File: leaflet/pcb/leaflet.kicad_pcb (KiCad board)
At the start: 2 copper layers, 99.1 x 48.3 mm, 34 parts, among them J1 Conn_01x02, J2 Conn_01x02, J3 USB_B_Micro, J4 Conn_01x14_Male, J5 Conn_01x14_Male, Q1 NTZD3155C, Q2 NTZD3155C, U1 MCP16252-I_CH, U2 MCP1711, U3 EFM32HG322F64G-B-QFP48, U4 IP4220CZ6, U5 NRF24L01_Breakout

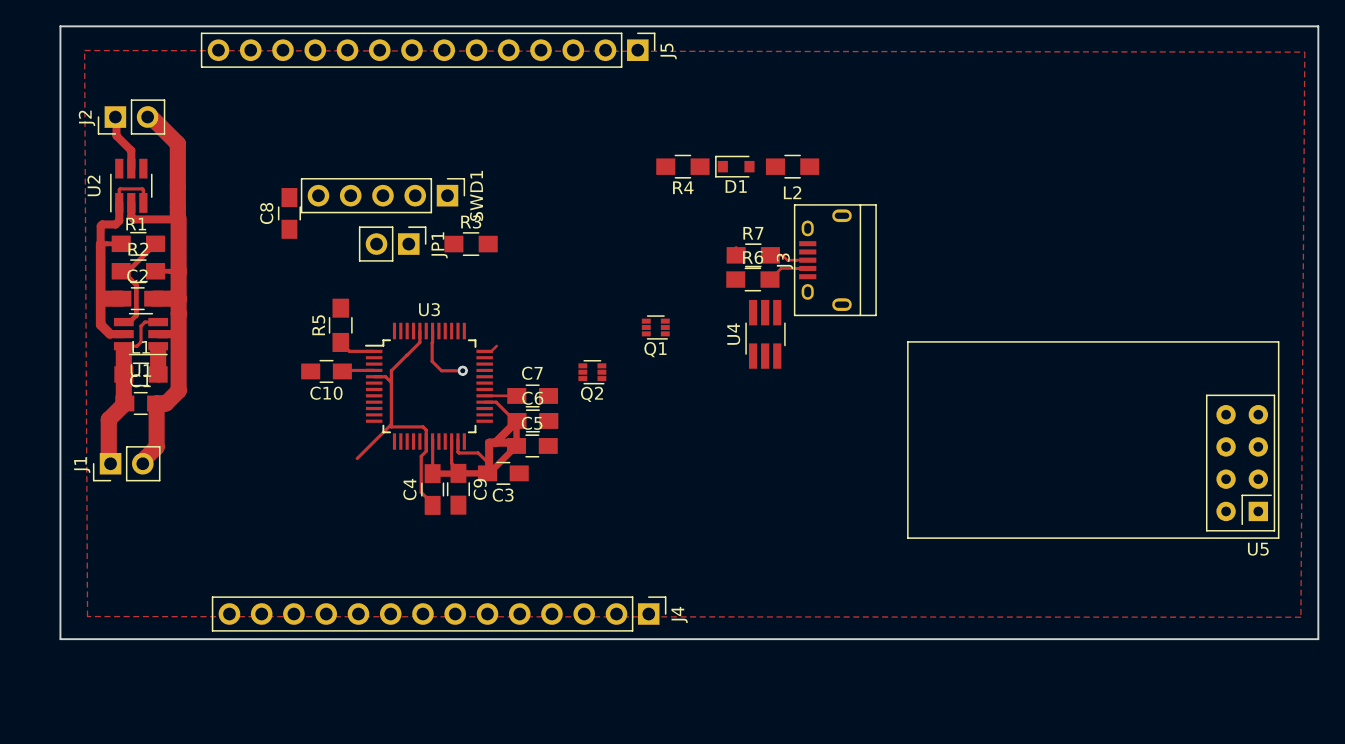
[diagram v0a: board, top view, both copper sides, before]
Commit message: stuff
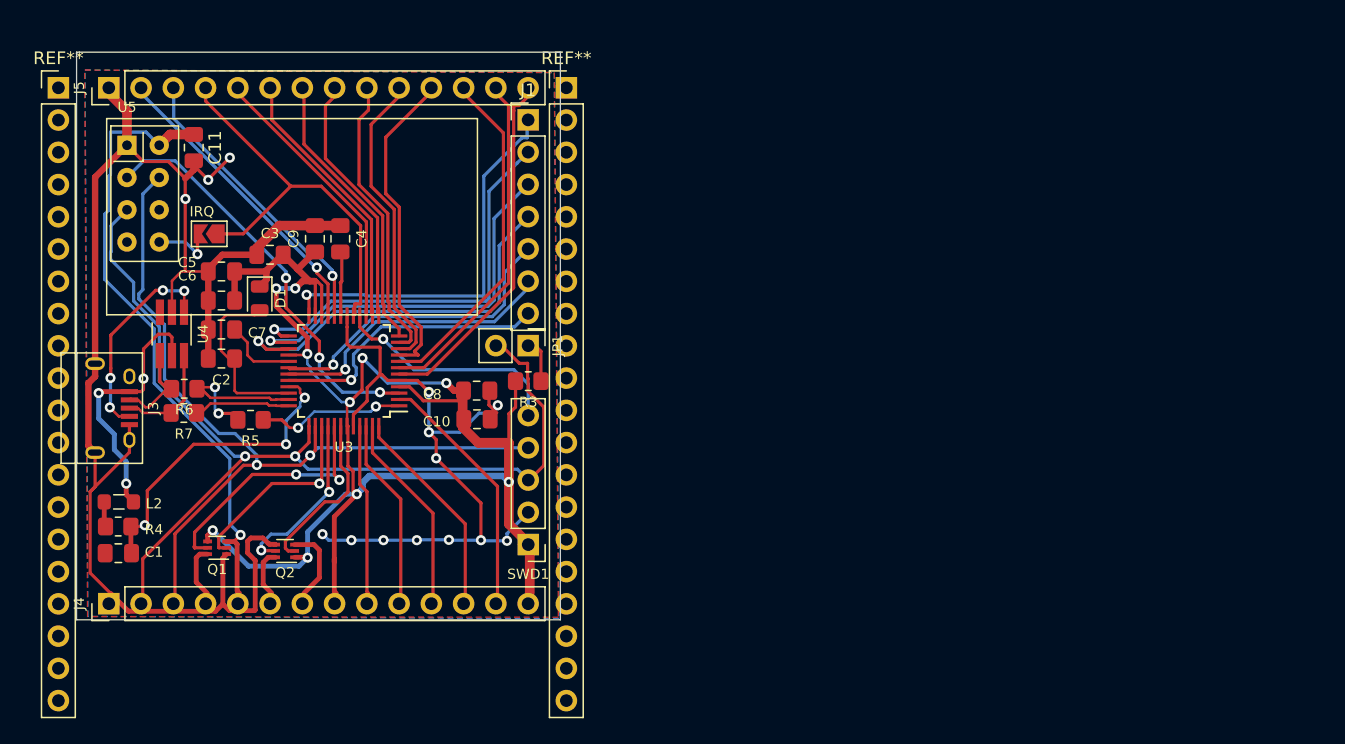
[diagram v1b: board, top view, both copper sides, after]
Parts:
- removed J2: Conn_01x02, Pin_Headers:Pin_Header_Straight_1x02_Pitch2.54mm
- removed L1: 4.7u, Inductors_SMD:L_0805_HandSoldering
- removed R1: 1.8M, Resistors_SMD:R_0805_HandSoldering
- removed R2: 1M, Resistors_SMD:R_0805_HandSoldering
- removed U1: MCP16252-I_CH, TO_SOT_Packages_SMD:SOT-23-6_Handsoldering
- removed U2: MCP1711, TO_SOT_Packages_SMD:SOT-23-6_Handsoldering
- added C11: 100n, Capacitor_SMD:C_0805_2012Metric_Pad1.18x1.45mm_HandSolder, F.Cu at (20.7, 19.7)
- added IRQ: Jumper_NO_Small, Jumper:SolderJumper-2_P1.3mm_Open_TrianglePad1.0x1.5mm, F.Cu at (21.9, 26.5)
- added REF**: PinHeader_1x20_P2.54mm_Vertical, Connector_PinHeader_2.54mm:PinHeader_1x20_P2.54mm_Vertical, F.Cu at (50.0, 15.0)
- added REF**: PinHeader_1x20_P2.54mm_Vertical, Connector_PinHeader_2.54mm:PinHeader_1x20_P2.54mm_Vertical, F.Cu at (10.0, 15.0)
- C1: value 10u -> 4.7u; footprint Capacitors_SMD:C_0805_HandSoldering -> Capacitor_SMD:C_0805_2012Metric_Pad1.18x1.45mm_HandSolder
- C10, C3, C4, C5, C6, C7, C8, C9: footprint Capacitors_SMD:C_0805_HandSoldering -> Capacitor_SMD:C_0805_2012Metric_Pad1.18x1.45mm_HandSolder
- C2: value 10u -> 1u; footprint Capacitors_SMD:C_0805_HandSoldering -> Capacitor_SMD:C_0805_2012Metric_Pad1.18x1.45mm_HandSolder
- D1: footprint Diodes_SMD:D_0805 -> Diode_SMD:D_0805_2012Metric
- J1: value Conn_01x02 -> Conn_01x06_Male; footprint Pin_Headers:Pin_Header_Straight_1x02_Pitch2.54mm -> Connector_PinHeader_2.54mm:PinHeader_1x07_P2.54mm_Vertical
- L2: footprint Inductors_SMD:L_0805_HandSoldering -> Inductor_SMD:L_0805_2012Metric_Pad1.05x1.20mm_HandSolder
- Q1, Q2: footprint Package_TO_SOT_SMD:SOT-563 -> 0_eurocad:SOT-563-slim
- R3, R4, R5, R6, R7: footprint Resistors_SMD:R_0805_HandSoldering -> Resistor_SMD:R_0805_2012Metric_Pad1.20x1.40mm_HandSolder
- moved U5 93.6 mm to (15.4, 19.5), turned to 0 degrees
- moved L2 59.3 mm to (14.8, 47.6)
- moved J3 57.3 mm to (14.2, 40.2), turned to 270 degrees
- moved R4 52.7 mm to (14.7, 49.5), turned to 0 degrees
- moved U4 46.7 mm to (18.9, 34.4), turned to 270 degrees
- moved R7 46.5 mm to (19.9, 40.6), turned to 180 degrees
- moved R6 45.6 mm to (19.9, 38.7), turned to 180 degrees
- moved J1 42.6 mm to (47.0, 17.5), turned to 0 degrees
- moved J4 42.5 mm to (14.0, 55.6), turned to 90 degrees
- moved J5 41.8 mm to (14.0, 15.0), turned to 90 degrees
- moved D1 38.9 mm to (25.9, 31.6), turned to 270 degrees
- moved Q1 38.7 mm to (22.5, 51.2)
- moved SWD1 28.2 mm to (47.0, 51.0), turned to 180 degrees
- moved C5 28.1 mm to (22.8, 29.5), turned to 180 degrees
- moved Q2 28.0 mm to (27.9, 51.5)
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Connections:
- net Net-(J3-Pad1) renamed /USB/VBUS
- net Net-(J3-Pad2) renamed /USB/DR-
- net Net-(J3-Pad3) renamed /USB/DR+
- net Net-(JP1-Pad1) renamed /Prog/I2C_PULLUP
- C1 pad 1: Vin -> USB_5v
- C2 pad 1: /power/Vsw -> USB_VREGO
- D1 pad 1: Net-(D1-Pad1) -> 3.3V
- D1 pad 2: /USB/USB_5V -> USB_VREGO
- J1 pad 1: Vin -> PD4
- J1 pad 2: GND -> PD5
- J4 pad 10: Net-(J4-Pad10) -> PE11
- J4 pad 11: Net-(J4-Pad11) -> PE12
- J4 pad 12: Net-(J4-Pad12) -> PE13
- J4 pad 13: Net-(J4-Pad13) -> PA1
- J4 pad 14: Net-(J4-Pad14) -> 3.3V
- J4 pad 2: Net-(J4-Pad2) -> USART1_SCK
- J4 pad 3: Net-(J4-Pad3) -> USART1_CS
- J4 pad 4: Net-(J4-Pad4) -> OUT_OD1
- J4 pad 5: Net-(J4-Pad5) -> AUX1_3.3V
- J4 pad 6: Net-(J4-Pad6) -> AUX2_3.3V
- J4 pad 7: Net-(J4-Pad7) -> OUT_OD2
- J4 pad 8: Net-(J4-Pad8) -> 3.3V
- J4 pad 9: Net-(J4-Pad9) -> PE10
- J5 pad 10: Net-(J5-Pad10) -> PC4
- J5 pad 11: Net-(J5-Pad11) -> PC3
- J5 pad 12: Net-(J5-Pad12) -> PC2
- J5 pad 13: Net-(J5-Pad13) -> I2C_SCL
- J5 pad 14: Net-(J5-Pad14) -> I2C_SDA
- J5 pad 2: Net-(J5-Pad2) -> USART0_CS
- J5 pad 3: Net-(J5-Pad3) -> USART0_CLK
- J5 pad 4: Net-(J5-Pad4) -> PB11
- J5 pad 5: Net-(J5-Pad5) -> PA10
- J5 pad 6: Net-(J5-Pad6) -> PA9
- J5 pad 7: Net-(J5-Pad7) -> PA8
- J5 pad 8: Net-(J5-Pad8) -> USART0_RX_MISO
- J5 pad 9: Net-(J5-Pad9) -> USART0_TX_MOSI
- JP1 pad 2: Net-(JP1-Pad2) -> USART1_SCK
- Q1 pad 3: Net-(Q1-Pad3) -> AUX1_3.3V
- R4 pad 1: Net-(D1-Pad1) -> /USB/USB_5V
- R4 pad 2: Vin -> USB_5v
- SWD1 pad 3: Net-(JP1-Pad2) -> USART1_SCK
- U3 pad 10: Net-(U3-Pad10) -> PC4
- U3 pad 11: Net-(U3-Pad11) -> USART0_TX_MOSI
- U3 pad 12: Net-(U3-Pad12) -> USART0_RX_MISO
- U3 pad 13: Net-(U3-Pad13) -> PA8
- U3 pad 14: Net-(U3-Pad14) -> PA9
- U3 pad 15: Net-(U3-Pad15) -> PA10
- U3 pad 17: Net-(U3-Pad17) -> PB11
- U3 pad 2: Net-(U3-Pad2) -> PA1
- U3 pad 20: Net-(U3-Pad20) -> USART0_CLK
- U3 pad 21: Net-(U3-Pad21) -> USART0_CS
- U3 pad 24: Net-(U3-Pad24) -> PD4
- U3 pad 25: (no net) -> PD5
- U3 pad 26: Net-(U3-Pad26) -> USART1_RX_MISO
- U3 pad 27: Net-(U3-Pad27) -> USART1_TX_MOSI
- U3 pad 30: Net-(U3-Pad30) -> PC8
- U3 pad 31: Net-(U3-Pad31) -> PC9
- U3 pad 32: Net-(U3-Pad32) -> PC10
- U3 pad 33: Net-(U3-Pad33) -> USB_5v
- U3 pad 34: Net-(U3-Pad34) -> USB_VREGO
- U3 pad 37: Net-(U3-Pad37) -> USART1_SCK
- U3 pad 38: Net-(U3-Pad38) -> USART1_CS
- U3 pad 45: Net-(U3-Pad45) -> PE10
- U3 pad 46: Net-(U3-Pad46) -> PE11
- U3 pad 47: Net-(U3-Pad47) -> PE12
- U3 pad 48: Net-(U3-Pad48) -> PE13
- U3 pad 6: Net-(U3-Pad6) -> I2C_SDA
- U3 pad 7: Net-(U3-Pad7) -> I2C_SCL
- U3 pad 8: Net-(U3-Pad8) -> PC2
- U3 pad 9: Net-(U3-Pad9) -> PC3
- U4 pad 3: Net-(U4-Pad3) -> (no net)
- U5 pad 2: AUX2_3.3V -> AUX1_3.3V
- U5 pad 6: USART1_MISO -> (no net)
- U5 pad 7: USART1_MOSI -> (no net)
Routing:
- net GND: track 63.8 -> 172.8 mm, vias 0 -> 14
- net 3.3V: track 37.4 -> 132.6 mm, vias 0 -> 10
- net USART1_SCK: track 0.00 -> 77.9 mm, vias 0 -> 2
- net USART1_CS: track 0.00 -> 65.7 mm, vias 0 -> 2
- net AUX1_3.3V: track 0.00 -> 50.0 mm, vias 0 -> 1
- net USART1_CE: track 0.00 -> 32.5 mm, vias 0 -> 3
- net PB11: track 0.00 -> 32.1 mm
- net PD5: track 0.00 -> 32.0 mm, vias 0 -> 1
- net USART1_TX_MOSI: track 0.00 -> 31.5 mm, vias 0 -> 1
- net PD4: track 0.00 -> 31.4 mm, vias 0 -> 1
- net USART1_RX_MISO: track 0.00 -> 31.4 mm, vias 0 -> 1
- net I2C_SDA: track 0.00 -> 27.8 mm
- net PC2: track 0.00 -> 26.6 mm
- net I2C_SCL: track 0.00 -> 26.6 mm
- net PC3: track 0.00 -> 25.3 mm
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- added copper zone on B.Cu, net GND
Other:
- board size 99.1 x 48.3 mm -> 38.1 x 44.7 mm
- net class Default: trace_width 0.25 -> 0.18
- rule pad_to_mask_clearance: 0.2 -> 0.05
